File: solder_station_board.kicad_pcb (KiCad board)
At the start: 2 copper layers, 49.5 x 44.2 mm, 40 parts, among them J1 RT_WELLER, J2 SERIAL, J3 PWR_15V, J4 PWR_5V, J5 VFD_DISPLAY, J6 ENCODER, J7 INPUT, P1 ISP, Q1 IRF9540, Q2 2N7002, U1 OPA343, U2 ATMEGA168-20AU

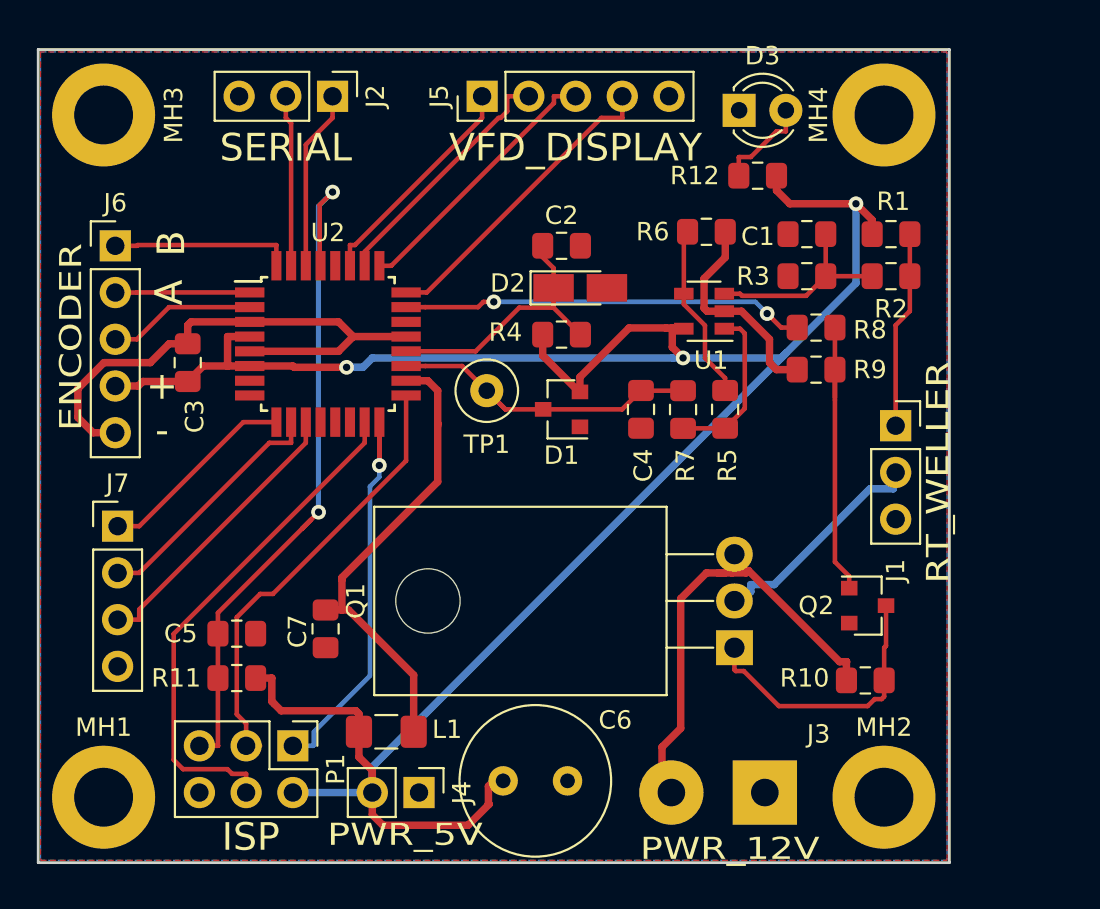
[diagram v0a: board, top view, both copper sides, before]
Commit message: two rt_weller
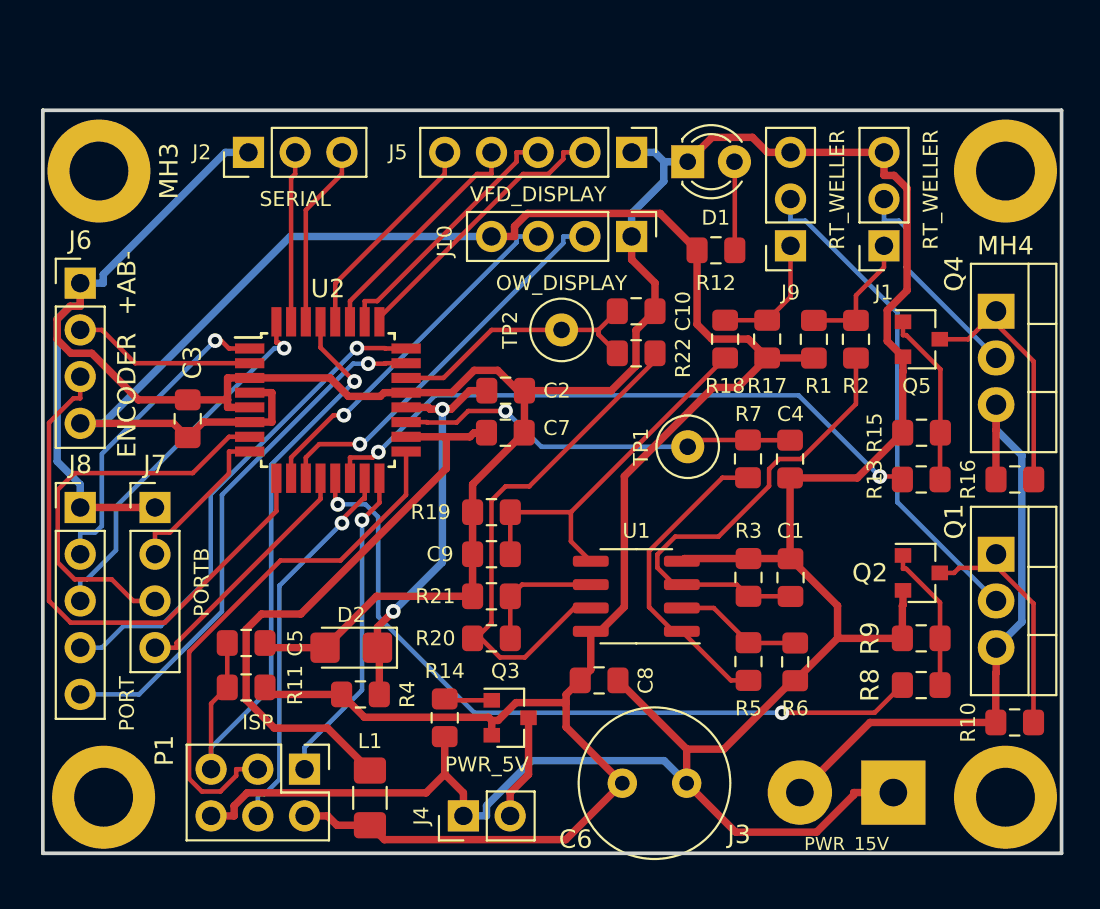
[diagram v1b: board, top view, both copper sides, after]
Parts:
- removed D3: LED_G, LED_THT:LED_D3.0mm
- added C10: 10n, Capacitor_SMD:C_0805_2012Metric_Pad1.15x1.40mm_HandSolder, F.Cu at (78.2, 47.9)
- added C8: 100n, Capacitor_SMD:C_0805_2012Metric_Pad1.15x1.40mm_HandSolder, F.Cu at (76.2, 68.0)
- added C9: 8n2, Capacitor_SMD:C_0805_2012Metric_Pad1.15x1.40mm_HandSolder, F.Cu at (70.3, 61.1)
- added G***: LOGO, custom_logo:pimium_paprika_7mm, B.Cu at (55.6, 45.9)
- added J10: OW_DISPLAY, Connector_PinHeader_2.54mm:PinHeader_1x04_P2.54mm_Vertical, F.Cu at (77.9, 43.8)
- added J8: PORT, Connector_PinHeader_2.54mm:PinHeader_1x05_P2.54mm_Vertical, F.Cu at (48.0, 58.6)
- added J9: RT_WELLER, Connector_PinSocket_2.54mm:PinSocket_1x03_P2.54mm_Vertical, F.Cu at (86.6, 44.3)
- added Q3: IRLM6401, Package_TO_SOT_SMD:SOT-23, F.Cu at (71.3, 70.0)
- added Q4: IRF9540, Package_TO_SOT_THT:TO-220-3_Vertical, F.Cu at (97.8, 47.9)
- added Q5: 2N7002, Package_TO_SOT_SMD:SOT-23, F.Cu at (93.7, 49.4)
- added R13: 1k, Resistor_SMD:R_0805_2012Metric_Pad1.15x1.40mm_HandSolder, F.Cu at (93.7, 57.0)
- added R14: 100K, Resistor_SMD:R_0805_2012Metric_Pad1.15x1.40mm_HandSolder, F.Cu at (67.8, 70.0)
- added R15: 2k2, Resistor_SMD:R_0805_2012Metric_Pad1.15x1.40mm_HandSolder, F.Cu at (93.7, 54.5)
- added R16: 4k7, Resistor_SMD:R_0805_2012Metric_Pad1.15x1.40mm_HandSolder, F.Cu at (98.8, 57.0)
- added R17: 10M, Resistor_SMD:R_0805_2012Metric_Pad1.15x1.40mm_HandSolder, F.Cu at (85.3, 49.4)
- added R18: 5k6, Resistor_SMD:R_0805_2012Metric_Pad1.15x1.40mm_HandSolder, F.Cu at (83.0, 49.4)
- added R19: 100k, Resistor_SMD:R_0805_2012Metric_Pad1.15x1.40mm_HandSolder, F.Cu at (70.3, 58.8)
- added R20: 39k, Resistor_SMD:R_0805_2012Metric_Pad1.15x1.40mm_HandSolder, F.Cu at (70.3, 65.7)
- added R21: 100, Resistor_SMD:R_0805_2012Metric_Pad1.15x1.40mm_HandSolder, F.Cu at (70.3, 63.4)
- added R22: 5k6, Resistor_SMD:R_0805_2012Metric_Pad1.15x1.40mm_HandSolder, F.Cu at (78.2, 50.2)
- added TP2: TEMP, TestPoint:TestPoint_Loop_D2.60mm_Drill0.9mm_Beaded, F.Cu at (74.1, 48.9)
- C1: value 10n -> 8n2
- D1: value BAT54S -> LED_G; footprint Package_TO_SOT_SMD:SOT-23 -> LED_THT:LED_D3.0mm
- D2: footprint Diode_SMD:D_MicroMELF_Hadsoldering -> Diode_SMD:D_1206_3216Metric_Castellated
- J6: footprint Connector_PinHeader_2.54mm:PinHeader_1x05_P2.54mm_Vertical -> Connector_PinHeader_2.54mm:PinHeader_1x04_P2.54mm_Vertical
- J7: value INPUT -> PORTB
- Q1: footprint Package_TO_SOT_THT:TO-220-3_Horizontal_TabDown -> Package_TO_SOT_THT:TO-220-3_Vertical
- R4: value 1k -> 560
- R5: value 68k -> 39k
- U1: value OPA343 -> OPA2343; footprint Package_TO_SOT_SMD:SOT-23-5 -> Package_SO:SOIC-8_3.9x4.9mm_P1.27mm
- moved R6 23.9 mm to (86.8, 67.0), turned to 270 degrees
- moved D2 23.2 mm to (62.7, 66.2), turned to 180 degrees
- moved R4 22.4 mm to (63.2, 68.7)
- moved R8 20.3 mm to (93.7, 68.2)
- moved C1 18.7 mm to (86.6, 62.4), turned to 90 degrees
- moved R3 16.7 mm to (84.3, 62.4), turned to 270 degrees
- moved U1 15.9 mm to (78.2, 63.4)
- moved R9 15.7 mm to (93.7, 65.7)
- moved D1 15.1 mm to (81.0, 39.8), turned to 0 degrees
- moved Q1 15.1 mm to (97.8, 61.1), turned to 270 degrees
- moved C7 14.5 mm to (71.1, 54.5), turned to 0 degrees
- moved R5 13.8 mm to (84.3, 66.9)
- moved TP1 11.3 mm to (81.0, 55.3)
- moved J1 9.80 mm to (91.7, 44.3), turned to 180 degrees
- moved J5 8.68 mm to (77.9, 39.3), turned to 270 degrees
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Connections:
- C4 pad 1: /TEMP -> /TEMP_L
- D1 pad 2: +5V -> Net-(D1-Pad2)
- J1 pad 2: Net-(J1-Pad2) -> /HEAT_L
- J2 pad 1: /RX -> GND
- J2 pad 3: GND -> /RX
- J4 pad 2: +5V -> Net-(J4-Pad2)
- J5 pad 1: /VFD_DATA -> GND
- J5 pad 2: /VFD_RCLK -> /~VFD_SRCLR
- J5 pad 4: /~VFD_SRCLR -> /VFD_RCLK
- J5 pad 5: GND -> /VFD_DATA
- J6 pad 1: /INP1 -> GND
- J6 pad 2: /INP2 -> /ENC_B
- J6 pad 3: /INP3 -> /ENC_A
- J7 pad 1: /INP4 -> GND
- J7 pad 2: /INP5 -> /PB7
- J7 pad 3: /INP6 -> /PB6
- J7 pad 4: GND -> /PB1
- Q1 pad 2: Net-(J1-Pad2) -> /HEAT_H
- R12 pad 1: Net-(D3-Pad2) -> Net-(D1-Pad2)
- R7 pad 1: /TEMP -> /TEMP_L
- R8 pad 1: /SOLDER -> /SOLDER_H
- TP1 pad 1: /TEMP -> /TEMP_L
- U1 pad 2: GND -> Net-(R5-Pad2)
- U1 pad 4: Net-(R5-Pad2) -> GND
- U1 pad 5: +5V -> Net-(C9-Pad1)
- U2 pad 1: /INP2 -> /PD3
- U2 pad 10: /INP5 -> /OW_DIO
- U2 pad 11: /INP6 -> /OW_RST
- U2 pad 12: (no net) -> /PB1
- U2 pad 13: (no net) -> /SOLDER_H
- U2 pad 14: (no net) -> /SOLDER_L
- U2 pad 19: /TEMP -> /TEMP_L
- U2 pad 2: /INP3 -> /ENC_B
- U2 pad 22: (no net) -> /TEMP_H
- U2 pad 23: /SOLDER -> /PC0
- U2 pad 24: /~VFD_SRCLR -> /PC1
- U2 pad 25: /VFD_SRCLK -> /~VFD_SRCLR
- U2 pad 26: /VFD_RCLK -> /VFD_SRCLK
- U2 pad 27: /VFD_DATA -> /VFD_RCLK
- U2 pad 28: (no net) -> /VFD_DATA
- U2 pad 32: /INP1 -> /PD2
- U2 pad 7: (no net) -> /PB6
- U2 pad 8: (no net) -> /PB7
- U2 pad 9: /INP4 -> /ENC_A
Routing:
- net GND: track 42.0 -> 234.1 mm
- net /SOLDER_H: track 0.00 -> 40.6 mm, vias 0 -> 2
- net /SOLDER_L: track 0.00 -> 34.4 mm, vias 0 -> 2
- net /ENC_A: track 0.00 -> 30.3 mm
- net /PC0: track 0.00 -> 28.9 mm, vias 0 -> 1
- net Net-(R20-Pad1): track 0.00 -> 28.2 mm
- net /PC1: track 0.00 -> 27.1 mm, vias 0 -> 1
- net /HEAT_H: track 0.00 -> 26.9 mm
- net /TEMP_L: track 0.00 -> 22.1 mm, vias 0 -> 1
- net /SOLDER: track 22.0 -> 0.00 mm, vias 2 -> 0
- net /PB6: track 0.00 -> 21.7 mm
- net /OW_RST: track 0.00 -> 21.5 mm, vias 0 -> 1
- net Net-(C9-Pad1): track 0.00 -> 20.5 mm
- net /PD2: track 0.00 -> 20.5 mm, vias 0 -> 1
- net /RST: track 56.0 -> 35.5 mm, vias 2 -> 1
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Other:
- board size 49.5 x 44.2 mm -> 55.4 x 40.4 mm
- board text added: "+AB-"
- board text removed: "+"
- board text removed: "-"
- board text removed: "A"
- board text removed: "B"
- board text removed: "ENCODER"
- board text removed: "ISP"
- board text removed: "PWR_12V"
- board text removed: "PWR_5V"
- board text removed: "RT_WELLER"
- board text removed: "SERIAL"
- board text removed: "VFD_DISPLAY"
